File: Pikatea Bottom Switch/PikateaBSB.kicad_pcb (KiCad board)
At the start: 2 copper layers, 20 parts, among them J1 Micro_SD_Card, J2 Conn_01x15, SW1 Rotary_Encoder_Switch, U1 AMS1117-3.3, U2 74LVC125APW,118

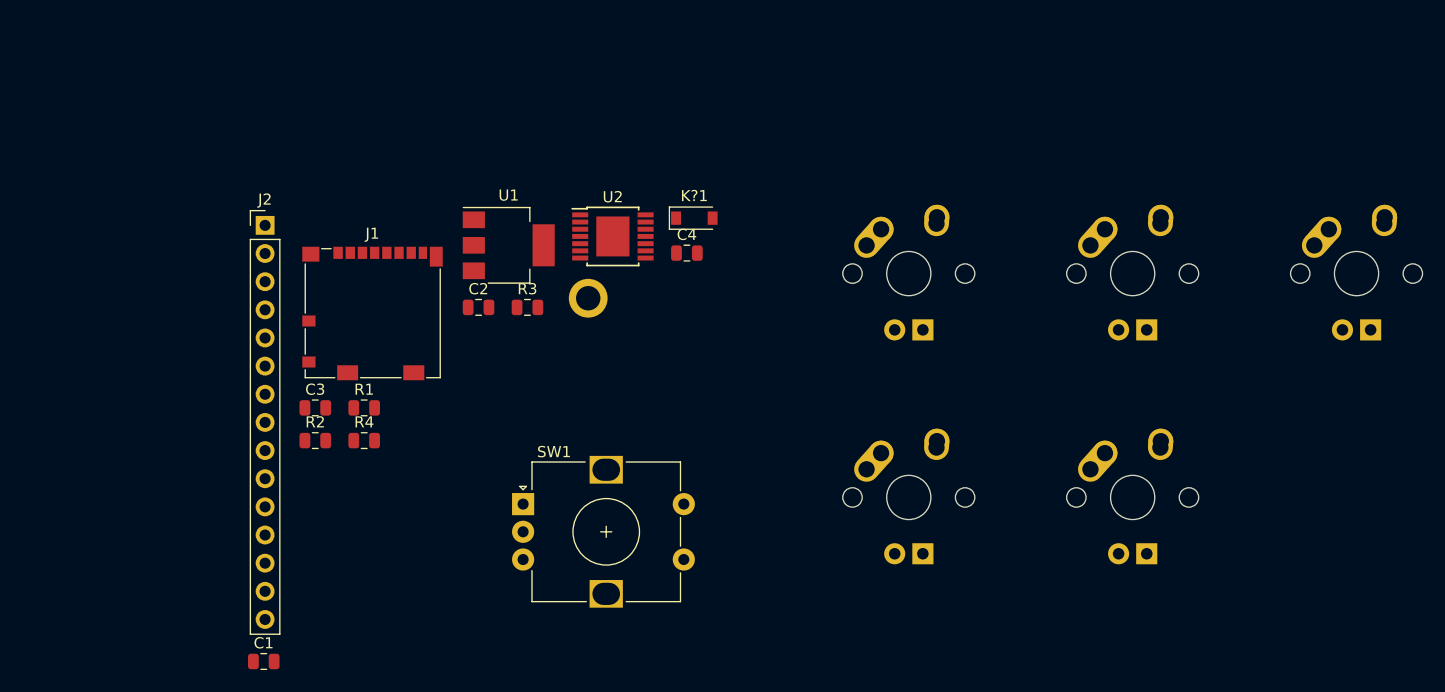
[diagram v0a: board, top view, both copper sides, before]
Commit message: rudimentary layout
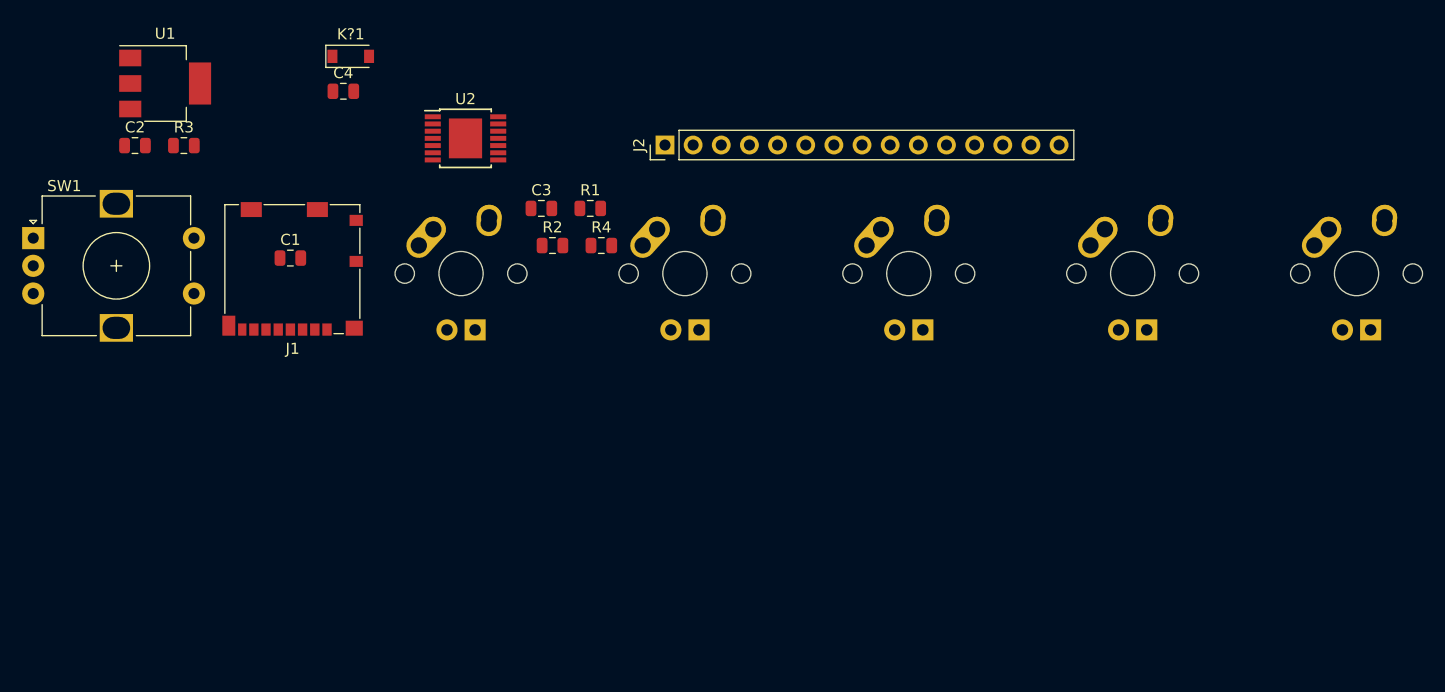
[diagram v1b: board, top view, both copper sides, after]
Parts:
- removed K?2: KEYSW, random-keyboard-parts:Generic-Mounthole
- moved SW1 50.3 mm to (115.2, 56.4)
- moved MX4 45.2 mm to (174.0, 59.6)
- moved MX2 45.2 mm to (153.8, 59.6)
- moved J2 36.8 mm to (172.2, 48.0), turned to 90 degrees
- moved C1 36.5 mm to (138.4, 58.2)
- moved C2 34.3 mm to (124.4, 48.0)
- moved C4 34.3 mm to (143.2, 43.1)
- moved K?1 34.3 mm to (143.8, 40.0)
- moved R3 34.3 mm to (128.8, 48.0)
- moved U1 34.3 mm to (127.1, 42.5)
- moved R2 27.7 mm to (162.1, 57.1)
- moved R4 27.7 mm to (166.5, 57.1)
- moved C3 27.2 mm to (161.1, 53.7)
- moved R1 27.2 mm to (165.5, 53.7)
- moved U2 16.0 mm to (154.2, 47.4)
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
